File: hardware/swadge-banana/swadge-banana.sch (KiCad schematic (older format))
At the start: 46 parts, among them J1 USB_B_Micro, Q1 Q_NPN_BEC, SW1 SW_SPDT, U1 ESP-13-WROOM-02D, U3 BUS_PCIexpress, U4 QMA6981, U5 AP1117-33, U6 OLED_CONNECTOR

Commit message: Update with my notional idea of what the banana swadge could be.
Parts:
- removed BT1, BT2: Battery, Swadge_Parts:2460, symbol Swadge_Parts:Battery
- removed C1, C17, C3: 0.1u, Swadge_Parts:C_0603_1608Metric, symbol Swadge_Parts:C
- removed C10, C2: 10u, Swadge_Parts:C_0603_1608Metric, symbol Swadge_Parts:C
- removed C16: 0.01u, Swadge_Parts:C_0603_1608Metric, symbol Swadge_Parts:C
- removed C18, C7: 2.2u, Swadge_Parts:C_0603_1608Metric, symbol Swadge_Parts:C
- removed C4, C5, C6, C9: 1u, Swadge_Parts:C_0603_1608Metric, symbol Swadge_Parts:C
- removed H1: Headband, Swadge_Parts:Headband, symbol Swadge_Parts:Headband
- removed LS1: Speaker, Swadge_Parts:Buzzer_12x9.5RM7.6, symbol Swadge_Parts:Speaker
- removed Q1: Q_NPN_BEC, Swadge_Parts:SOT-23, symbol Swadge_Parts:Q_NPN_BEC
- removed R1, R2, R3, R4: 10K, Swadge_Parts:R_0603_1608Metric, symbol Swadge_Parts:R_US
- removed R5: 70, Swadge_Parts:R_0603_1608Metric, symbol Swadge_Parts:R_US
- removed R6: 390k, Swadge_Parts:R_0603_1608Metric, symbol Swadge_Parts:R_US
- removed R7: 100, Swadge_Parts:R_0603_1608Metric, symbol Swadge_Parts:R_US
- removed S1: 4-1437565-2, Swadge_Parts:SW_4-1437565-2, symbol Swadge_Parts:4-1437565-2
- removed S2, S3: B3FS-4002P, Swadge_Parts:B3FS4002P, symbol Swadge_Parts:B3FS-4002P
- removed SW1: SW_SPDT, Swadge_Parts:SW_SPDT_PCM12, symbol Swadge_Parts:SW_SPDT
- removed U1: ESP-13-WROOM-02D, Swadge_Parts:ESP-13-WROOM-02, symbol Swadge_Parts:ESP-13-WROOM-02D
- removed U4: QMA6981, Swadge_Parts:QMA6981, symbol Swadge_Parts:QMA6981
- removed U5: AP1117-33, Swadge_Parts:SOT-223-3_TabPin2, symbol Swadge_Parts:AP2114H-3.3TRG1
- removed U6: OLED_CONNECTOR, Swadge_Parts:microbuilder-UG-2864HSWEG01_0.96IN_WRAPAROUND, symbol Swadge_Parts:OLED_CONNECTOR
- added C? (x2): 10u, Swadge_Parts:C_0603_1608Metric, symbol Swadge_Parts:C
- added C? (x3): 0.1u, Swadge_Parts:C_0603_1608Metric, symbol Swadge_Parts:C
- added C? (x2): 1u, Swadge_Parts:C_0603_1608Metric, symbol Swadge_Parts:C
- added C? (x2): 0.22u, Swadge_Parts:C_0603_1608Metric, symbol Swadge_Parts:C
- added C?: 0.047uF, Swadge_Parts:C_0603_1608Metric, symbol Swadge_Parts:C
- added MK?: Microphone, Swadge_Parts:CMA-4544PF-W, symbol Swadge_Parts:Microphone
- added Q? (x2): Q_NPN_BEC, Swadge_Parts:SOT-23, symbol Swadge_Parts:Q_NPN_BEC
- added R? (x5): 10K, Swadge_Parts:R_0603_1608Metric, symbol Swadge_Parts:R_US
- added R?: 220k, Swadge_Parts:R_0603_1608Metric, symbol Swadge_Parts:R_US
- added R? (x2): 47K, Swadge_Parts:R_0603_1608Metric, symbol Swadge_Parts:R_US
- added R?: 470, Swadge_Parts:R_0603_1608Metric, symbol Swadge_Parts:R_US
- added R?: 3.9k, Swadge_Parts:R_0603_1608Metric, symbol Swadge_Parts:R_US
- added S? (x5): B3FS-4002P_PROGRAM, Swadge_Parts:B3FS4002P, symbol Swadge_Parts:B3FS-4002P
- added S?: B3FS-4002P_REST, Swadge_Parts:B3FS4002P, symbol Swadge_Parts:B3FS-4002P
- added U?: CP2102N-A01-GQFN24, Swadge_Parts:QFN-24-1EP_4x4mm_P0.5mm_EP2.6x2.6mm, symbol Swadge_Parts:CP2102N-A01-GQFN24
- added U?: MCP6001UT-I_OT, Swadge_Parts:SOT-23-5, symbol Swadge_Parts:MCP6001UT-I_OT
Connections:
- net labels added: AUD_VCC, DTR_GPIO0, RTS_EN
- wire segments 211 -> 148
- no-connect marks 12 -> 4
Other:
- note added: "AUD_PWR is actually our "free" pin."
- note added: "Mic Circuit"
- note added: "PCB must be 1.6mm\nthick for optimal\nbananing\n\nUses regulator on\nswadge."
- note added: "RESET / PGM Logic"
- note added: "THIS SECTION IS JUST NOTIONAL"
- note added: "TODO:\n * Consider using 5V for LEDs."
- note added: "Target Transition:\n1) 62.5 us + 31.25 us = 93.75 us || 3.9k/.033uF\n2) 187.5 us + 31.25 us = 218.75 us || 3.9k/.082uF\n3) 562.5 us + 31.25 us = 593.75 us || 3.9k/.22uF\n4) 1687.5 us + 31.25 us = 1718.75 us || 3.9k/.680uF\n\nNominal button scan rate: 250 Hz.\n\nTODO: Breadboard circuit. \nTune 3.9k resistor depending on TTL/CMOS props of ESP.\n\nNOTE: Pin can still be used for other mid-speed I/O."
- note added: "USB Programming"
- note added: "Use precision parts!"
- note removed: "Accelerometer Circuit"
- note removed: "Boot Resistors"
- note removed: "Buttons"
- note removed: "Buzzer"
- note removed: "Display Circuit"
- note removed: "ESP8266 Circuit"
- note removed: "GPIO0 is pulled high to boot\nnormally and low to enter\nUART programming mode"
- note removed: "I2C Address 0x78\nw/ SA0 at GND"
- note removed: "If GPIO2 is low and GPIO15\nis high it will boot in\nSD-Card mode"
- note removed: "Left"
- note removed: "Menu"
- note removed: "PCB must be 1.6mm\nthick for PCIe"
- note removed: "Power Circuit"
- note removed: "Pullups are in the\nboot resistor"
- note removed: "Right"
- note removed: "The resistors on SDA and SCL\nboth configure boot and are\npullups for I2C"
- moved on the sheet: J1

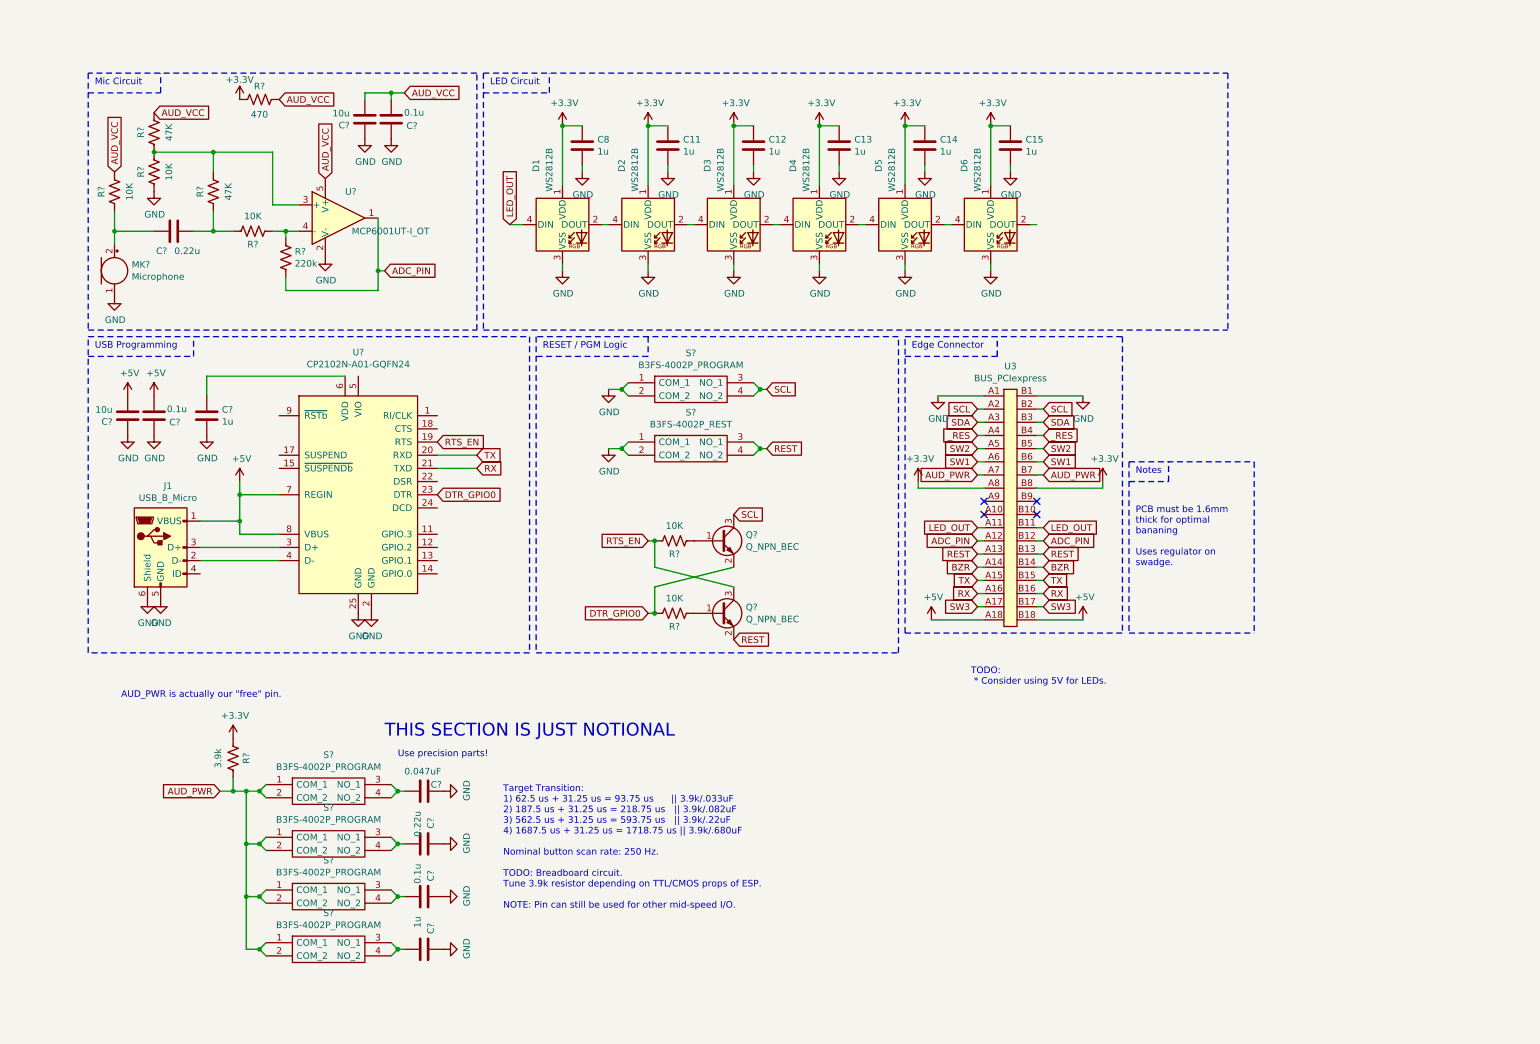
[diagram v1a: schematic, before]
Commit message: Add my notional banana
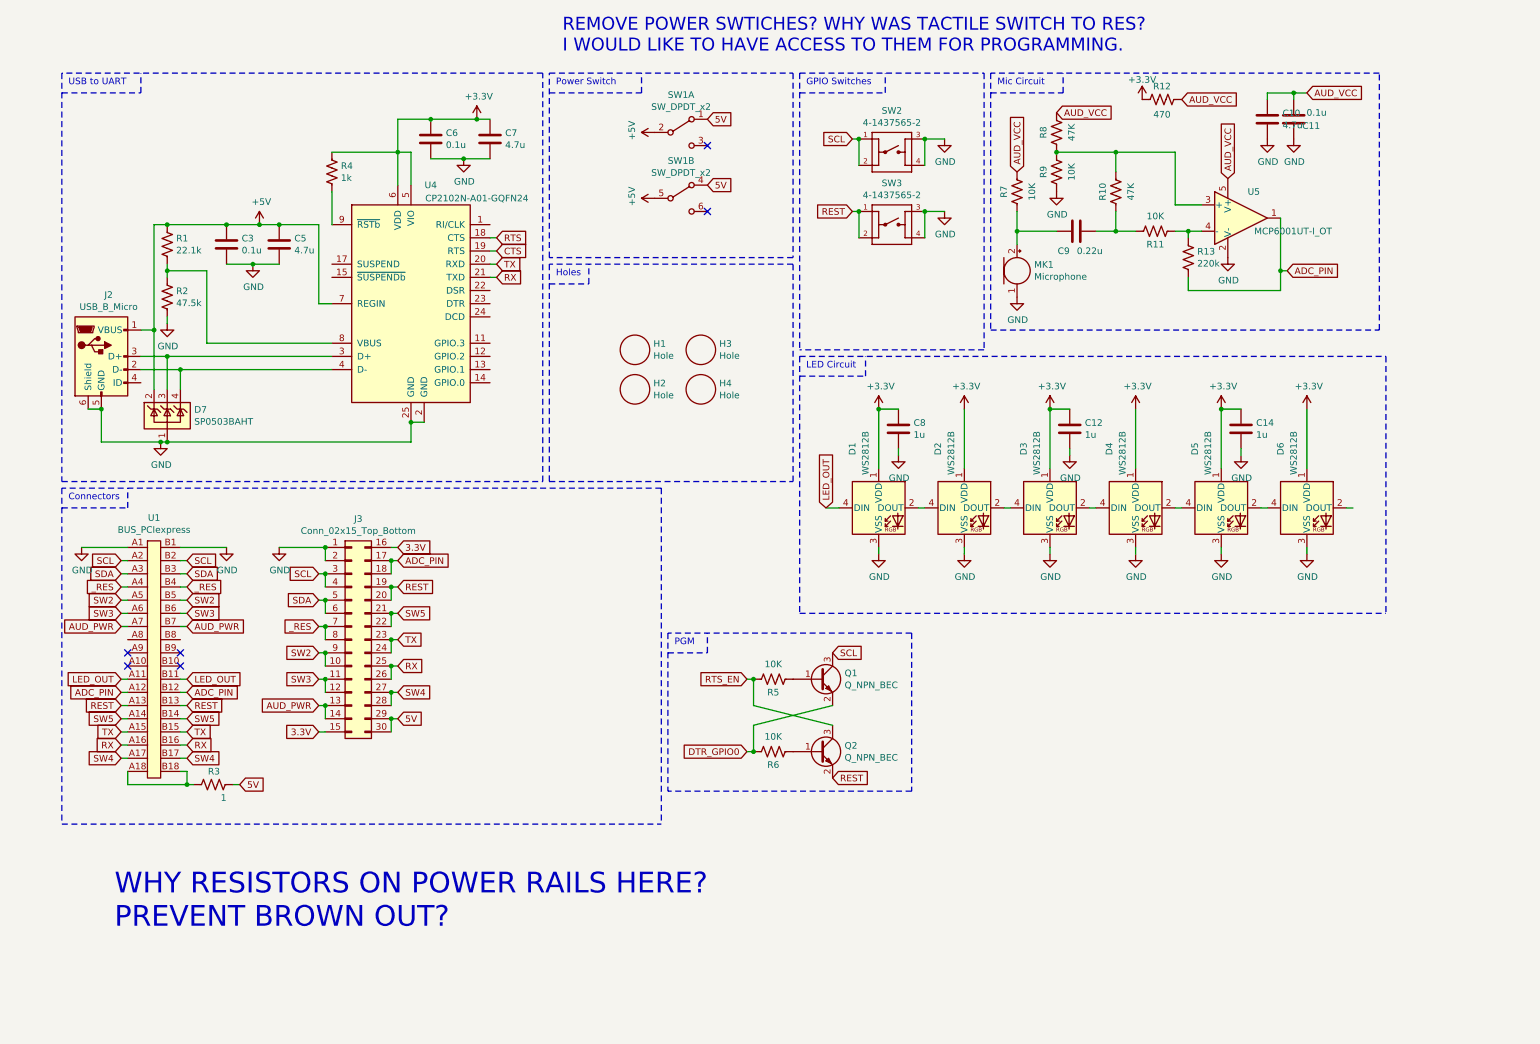
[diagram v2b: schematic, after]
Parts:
- removed C11, C13, C15, C? (x2): 1u, Swadge_Parts:C_0603_1608Metric, symbol Swadge_Parts:C
- removed C? (x2): 10u, Swadge_Parts:C_0603_1608Metric, symbol Swadge_Parts:C
- removed C? (x2): 0.1u, Swadge_Parts:C_0603_1608Metric, symbol Swadge_Parts:C
- removed C?: 0.047uF, Swadge_Parts:C_0603_1608Metric, symbol Swadge_Parts:C
- removed C?: 0.22u, Swadge_Parts:C_0603_1608Metric, symbol Swadge_Parts:C
- removed J1: USB_B_Micro, Swadge_Parts:USB_Micro-B_Molex_47346-0001, symbol Swadge_Parts:USB_B_Micro
- removed R?: 3.9k, Swadge_Parts:R_0603_1608Metric, symbol Swadge_Parts:R_US
- removed S? (x5): B3FS-4002P_PROGRAM, Swadge_Parts:B3FS4002P, symbol Swadge_Parts:B3FS-4002P
- removed S?: B3FS-4002P_REST, Swadge_Parts:B3FS4002P, symbol Swadge_Parts:B3FS-4002P
- removed U3: BUS_PCIexpress, Swadge_Parts:BUS_PCIexpress, symbol Swadge_Parts:BUS_PCIexpress
- removed U?: CP2102N-A01-GQFN24, Swadge_Parts:QFN-24-1EP_4x4mm_P0.5mm_EP2.6x2.6mm, symbol Swadge_Parts:CP2102N-A01-GQFN24
- added C10, C5, C7: 4.7u, Swadge_Parts:C_0603_1608Metric, symbol Swadge_Parts:C
- added C3, C6: 0.1u, Swadge_Parts:C_0603_1608Metric, symbol Swadge_Parts:C
- added D7: SP0503BAHT, Swadge_Parts:SOT-143, symbol Swadge_Parts:SP0503BAHT
- added H1, H2, H3, H4: Hole, Swadge_Parts:Hole, symbol Swadge_Parts:Hole
- added J2: USB_B_Micro, Swadge_Parts:USB_Micro-B_Molex_47346-0001, symbol Swadge_Parts:USB_B_Micro
- added J3: Conn_02x15_Top_Bottom, Swadge_Parts:PinHeader_2x15_P2.54mm_Vertical, symbol Swadge_Parts:Conn_02x15_Top_Bottom
- added R1: 22.1k, Swadge_Parts:R_0603_1608Metric, symbol Swadge_Parts:R_US
- added R2: 47.5k, Swadge_Parts:R_0603_1608Metric, symbol Swadge_Parts:R_US
- added R3: 1, Swadge_Parts:R_Axial_DIN0207_L6.3mm_D2.5mm_P10.16mm_Horizontal, symbol Swadge_Parts:R_US
- added R4: 1k, Swadge_Parts:R_0603_1608Metric, symbol Swadge_Parts:R_US
- added SW1: SW_DPDT_x2, Swadge_Parts:JS202011CQN, symbol Swadge_Parts:SW_DPDT_x2
- added SW2, SW3: 4-1437565-2, Swadge_Parts:SW_4-1437565-2, symbol Swadge_Parts:4-1437565-2
- added U1: BUS_PCIexpress, Swadge_Parts:10018784-10210TLF, symbol Swadge_Parts:BUS_PCIexpress
- added U4: CP2102N-A01-GQFN24, Swadge_Parts:QFN-24-1EP_4x4mm_P0.5mm_EP2.6x2.6mm, symbol Swadge_Parts:CP2102N-A01-GQFN24
- gave numbers to parts that had none: 15
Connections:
- net +3V3: now also C6.1, C7.1, R4.2, U4.5 (VIO), U4.6 (VDD)
- net +5V: now also C3.1, C5.1, D7.2 (K), J2.1 (VBUS), R1.1, SW1.2 (B), SW1.5 (B), U4.7 (REGIN)
- net ADC_PIN: now also J3.17 (Pin_17), J3.18 (Pin_18), U1.A12, U1.B12
- net AUD_PWR: now also J3.13 (Pin_13), J3.14 (Pin_14), U1.A7, U1.B7
- net AUD_VCC: now also C10.1
- net GND: now also C10.2, C3.2, C5.2, C6.2, C7.2, D7.1 (A), J2.5 (GND), J2.6 (Shield), J3.1 (Pin_1), J3.2 (Pin_2), R2.2, SW2.3, SW2.4, SW3.3, SW3.4, U1.A1, U1.B1, U4.2 (GND), U4.25 (GND)
- net LED_OUT: now also U1.A11, U1.B11
- net REST: now also J3.19 (Pin_19), J3.20 (Pin_20), SW3.1, SW3.2, U1.A13, U1.B13
- net RX: now also J3.25 (Pin_25), J3.26 (Pin_26), U1.A16, U1.B16, U4.21 (TXD)
- net SCL: now also J3.3 (Pin_3), J3.4 (Pin_4), SW2.1, SW2.2, U1.A2, U1.B2
- net SDA: now also J3.5 (Pin_5), J3.6 (Pin_6), U1.A3, U1.B3
- net SW2: now also J3.10 (Pin_10), J3.9 (Pin_9), U1.A5, U1.B5
- net SW3: now also J3.11 (Pin_11), J3.12 (Pin_12), U1.A6, U1.B6
- net TX: now also J3.23 (Pin_23), J3.24 (Pin_24), U1.A15, U1.B15, U4.20 (RXD)
- net _RES: now also J3.7 (Pin_7), J3.8 (Pin_8), U1.A4, U1.B4
- new net: R3.1, U1.A18, U1.B18
- new net: D7.3 (K), J2.3 (D+), U4.3 (D+)
- new net: D7.4 (K), J2.2 (D-), U4.4 (D-)
- new net: R1.2, R2.1, U4.8 (VBUS)
- new net: R4.1, U4.9 (~RSTb)
- new net 3.3V: J3.15 (Pin_15), J3.16 (Pin_16)
- new net 5V: J3.29 (Pin_29), J3.30 (Pin_30), R3.2, SW1.1 (A), SW1.4 (A)
- new net CTS: U4.19 (RTS)
- new net RTS: U4.18 (CTS)
- new net SW4: J3.27 (Pin_27), J3.28 (Pin_28), U1.A17, U1.B17
- new net SW5: J3.21 (Pin_21), J3.22 (Pin_22), U1.A14, U1.B14
- no-connect marks 4 -> 6
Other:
- note added: "Connectors"
- note added: "GPIO Switches"
- note added: "Holes"
- note added: "PGM"
- note added: "Power Switch"
- note added: "REMOVE POWER SWTICHES? WHY WAS TACTILE SWITCH TO RES?\nI WOULD LIKE TO HAVE ACCESS TO THEM FOR PROGRAMMING."
- note added: "USB to UART"
- note added: "WHY RESISTORS ON POWER RAILS HERE?\nPREVENT BROWN OUT?"
- note removed: "AUD_PWR is actually our "free" pin."
- note removed: "Edge Connector"
- note removed: "Notes"
- note removed: "PCB must be 1.6mm\nthick for optimal\nbananing\n\nUses regulator on\nswadge."
- note removed: "RESET / PGM Logic"
- note removed: "THIS SECTION IS JUST NOTIONAL"
- note removed: "TODO:\n * Consider using 5V for LEDs."
- note removed: "Target Transition:\n1) 62.5 us + 31.25 us = 93.75 us || 3.9k/.033uF\n2) 187.5 us + 31.25 us = 218.75 us || 3.9k/.082uF\n3) 562.5 us + 31.25 us = 593.75 us || 3.9k/.22uF\n4) 1687.5 us + 31.25 us = 1718.75 us || 3.9k/.680uF\n\nNominal button scan rate: 250 Hz.\n\nTODO: Breadboard circuit. \nTune 3.9k resistor depending on TTL/CMOS props of ESP.\n\nNOTE: Pin can still be used for other mid-speed I/O."
- note removed: "USB Programming"
- note removed: "Use precision parts!"
- moved on the sheet: C11, C12, C14, C8, C9, D1, D2, D3, D4, D5, D6, MK1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
